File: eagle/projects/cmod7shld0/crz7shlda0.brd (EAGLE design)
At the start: 30.5 x 67.7 mm, 26 parts, among them Q1 BSS138, Q2 BSS138, Q3 BSS138, Q4 BSS138

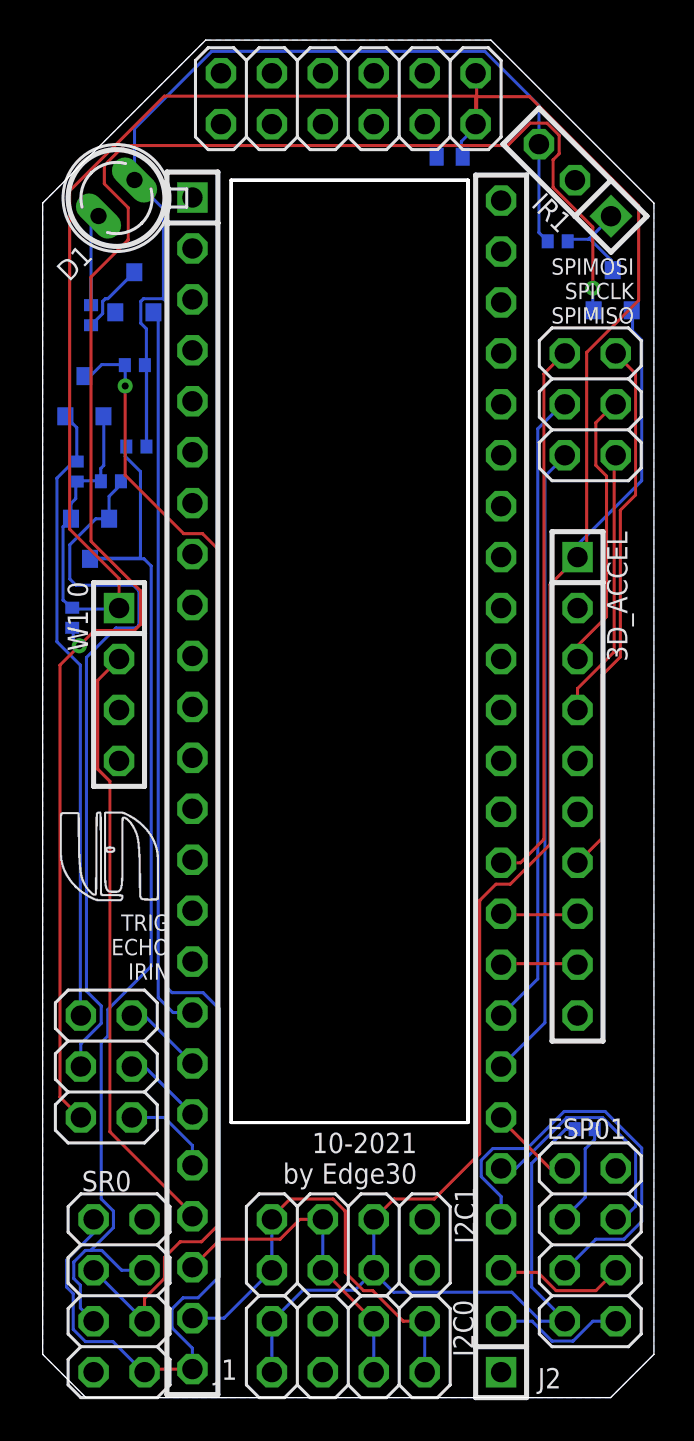
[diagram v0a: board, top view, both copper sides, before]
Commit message: cmod7shld0, crz7shlda0 production
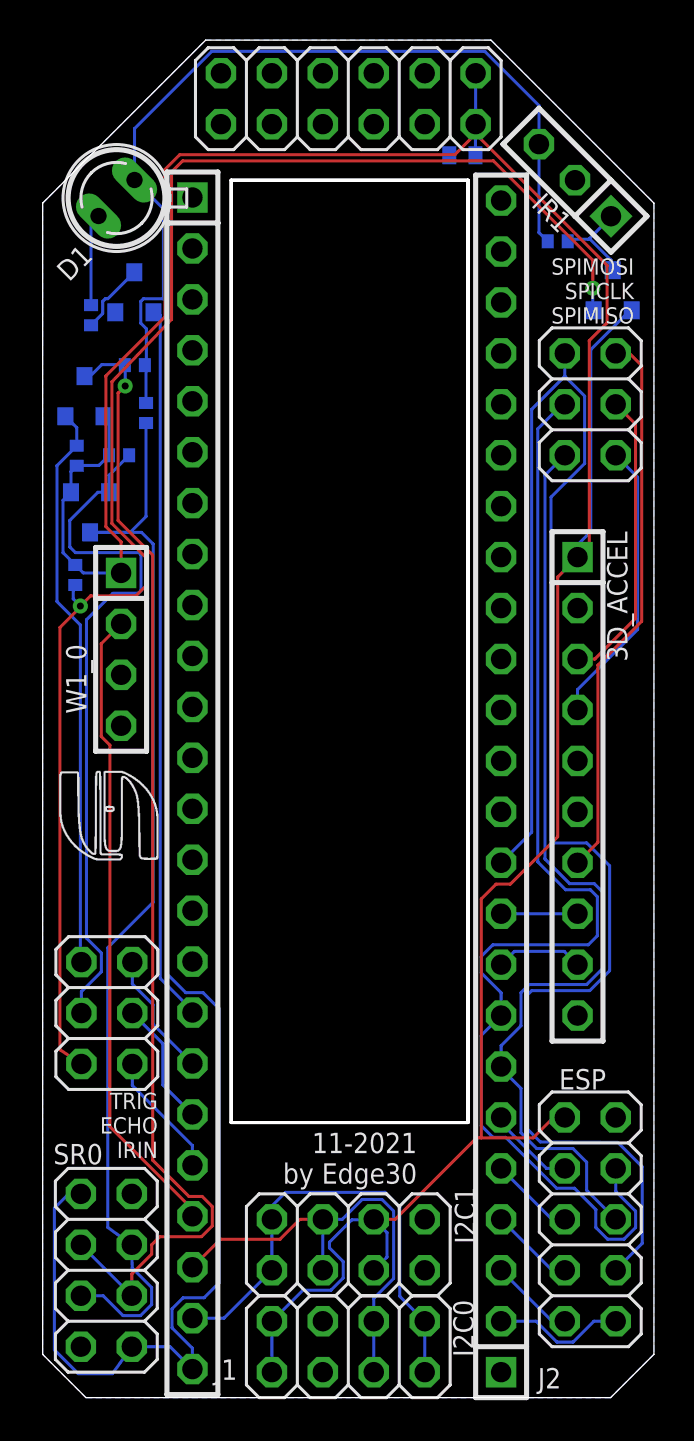
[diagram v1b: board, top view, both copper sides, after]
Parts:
- removed ESP01: (no value), pinhead:2X04
- removed R2: 10k, rcl:R0402
- added ESP: NA, pinhead:2X05
- 3D_ACCEL, IR1, J1, J2, JP0, JP1, PMOD0, SR0, W1_0: value (none) -> NA
- I2C0: value (none) -> I2C
- I2C1: value (none) -> I2Crev
- moved JP1 2.67 mm to (3.20, 19.2)
- moved R4 2.14 mm to (1.63, 41.0)
- moved W1_0 1.76 mm to (3.91, 37.3)
- moved R5 1.74 mm to (5.16, 49.1), turned to 90 degrees
- moved SR0 1.42 mm to (3.17, 6.35)
- moved R6 1.36 mm to (3.81, 47.0)
- moved Q3 1.32 mm to (2.36, 44.1)
- moved R8 0.79 mm to (1.70, 47.0)
- moved C1 0.64 mm to (20.9, 62.0)
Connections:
- removed net GPO0: ESP01.6, J2.3
- removed net GPO2: ESP01.4, J2.5
- removed net KCHIP_EN: ESP01.3, R2.2
- removed net URST: ESP01.5, J2.4
- removed net URXD: ESP01.8, J2.2
- removed net UTXD: ESP01.1, J2.6
- new net CS_ESP: ESP.1, J2.2
- new net EN_ESP: ESP.4, J2.4
- new net GPIO3: ESP.8, J2.6
- new net GPIO8: ESP.2, J2.3
- new net GPIO9: ESP.6, J2.5
- net K3V: now also ESP.10; no longer ESP01.7, R2.1
- net KGND: now also ESP.9; no longer ESP01.2
- net SPI_CLK: now also ESP.7
- net SPI_MISO: now also ESP.5
- net SPI_MOSI: now also ESP.3
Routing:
- net SPI_MOSI: track 27.3 -> 83.1 mm
- net K3V: track 179.3 -> 150.0 mm
- net SPI_CLK: track 31.9 -> 58.7 mm
- net URST: track 21.6 -> 0.00 mm
- net SPI_MISO: track 31.9 -> 47.7 mm
- net GPO2: track 12.5 -> 0.00 mm
- net IR_IN_: track 87.5 -> 77.1 mm
- net GPO0: track 6.62 -> 0.00 mm
- net CS_ESP: track 0.00 -> 6.58 mm
- net URXD: track 6.54 -> 0.00 mm
- net KSCL: track 16.3 -> 22.7 mm
- net KCHIP_EN: track 5.11 -> 0.00 mm
- net GPIO3: track 0.00 -> 4.39 mm
- net UTXD: track 4.29 -> 0.00 mm
- net EN_ESP: track 0.00 -> 4.23 mm
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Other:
- board text added: "11-2021 by Edge30"
- board text removed: "10-2021 by Edge30"
